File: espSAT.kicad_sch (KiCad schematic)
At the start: 20 parts, among them J1 Micro_SD_Card_Det2, J2 Prog, J3 C5, J4 C1, J5 C2, J6 C6, U1 ESP32-WROOM-32, U3 AZ1117-3.3, U4 AZ1117-3.3

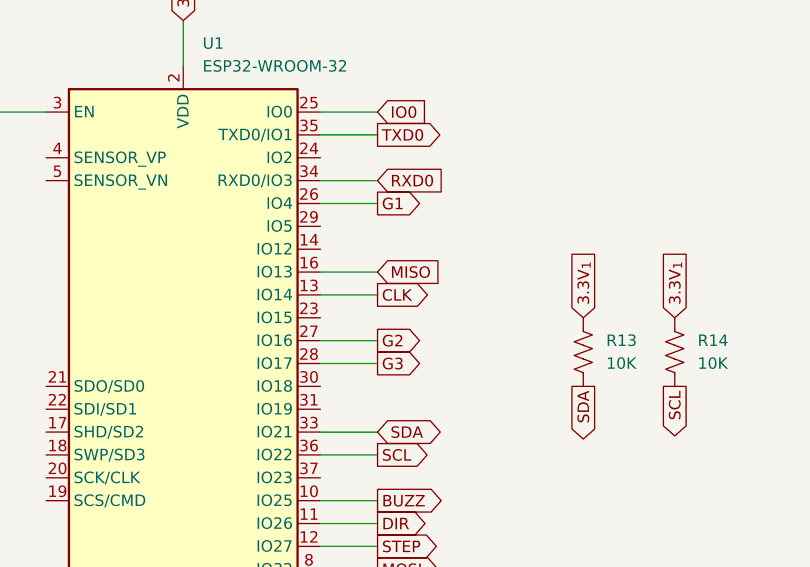
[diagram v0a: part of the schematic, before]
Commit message: v1.2
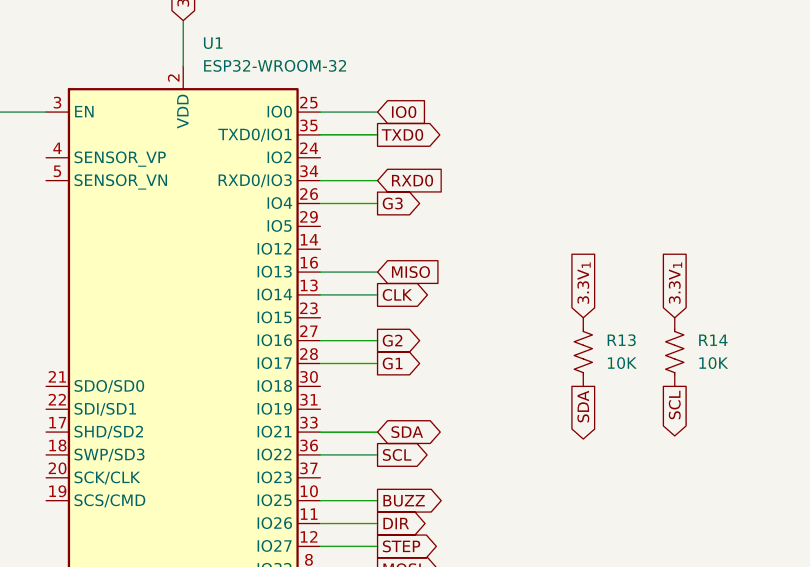
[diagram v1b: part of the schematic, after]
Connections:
- net G1: now also U1.28 (IO17); no longer U1.26 (IO4)
- net G3: now also U1.26 (IO4); no longer U1.28 (IO17)
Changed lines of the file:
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@@
 	(global_label "G3"
 		(shape output)
-		(at 88.9 134.62 0)
+		(at 88.9 116.84 0)
 		(fields_autoplaced yes)
 		(effects
@@
 		)
 		(property "Intersheetrefs" "${INTERSHEET_REFS}"
-			(at 94.3647 134.62 0)
+			(at 94.3647 116.84 0)
 			(effects
 				(font
@@
 	(global_label "G1"
 		(shape output)
-		(at 88.9 116.84 0)
+		(at 88.9 134.62 0)
 		(fields_autoplaced yes)
 		(effects
@@
 		)
 		(property "Intersheetrefs" "${INTERSHEET_REFS}"
-			(at 94.3647 116.84 0)
+			(at 94.3647 134.62 0)
 			(effects
 				(font
